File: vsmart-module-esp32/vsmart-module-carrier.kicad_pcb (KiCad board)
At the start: 2 copper layers, 105 x 82 mm, 12 parts, among them J1 EXTERNAL 5V INPUT, J2 EXTERNAL 5V 2A SIM INPUT, U1 ESP32-DevKitC 38-pin, U2 MPU6050 GY-521 MODULE, U3 GPS NEO-7M GY-GPSU3, U4 A7680C TDM2309 4G

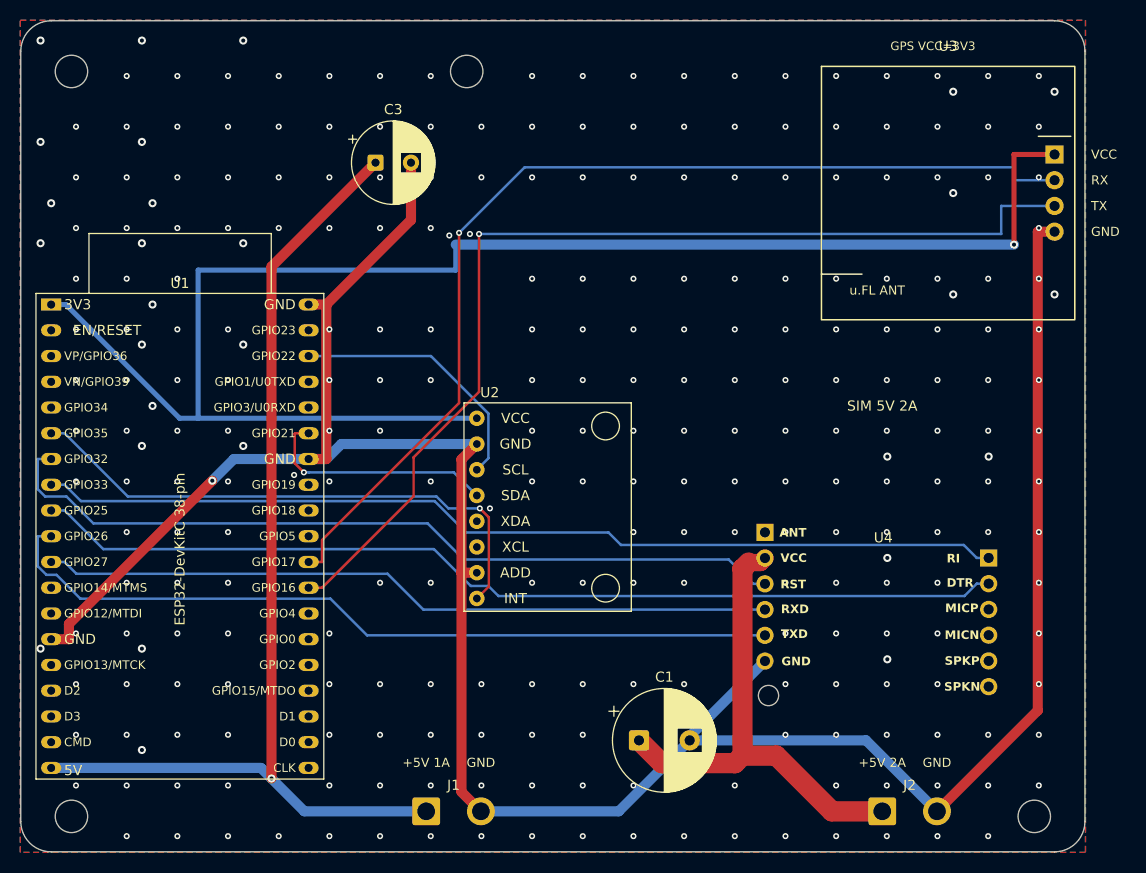
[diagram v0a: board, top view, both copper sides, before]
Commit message: chore: sync full workspace source into monorepo
Push current state of all first-party Vsmart components (backend, web,
web mobile, infrastructure, firmware, hardware, osrm, module variants)
directly from the DATN working tree, which is now the root of this repo.

Excluded: DRC/audit/build reports, auto-generated PCB snapshots, OSRM map
data, dependencies (node_modules/.venv/Pods/.pio), device secrets/certs,
.env files, local agent tooling, and vendored third-party reference repos
(ESP32_OSM_NAV, AWS guidance sample) per CLAUDE.md.

Co-Authored-By: Claude Sonnet 5 <noreply@anthropic.com>
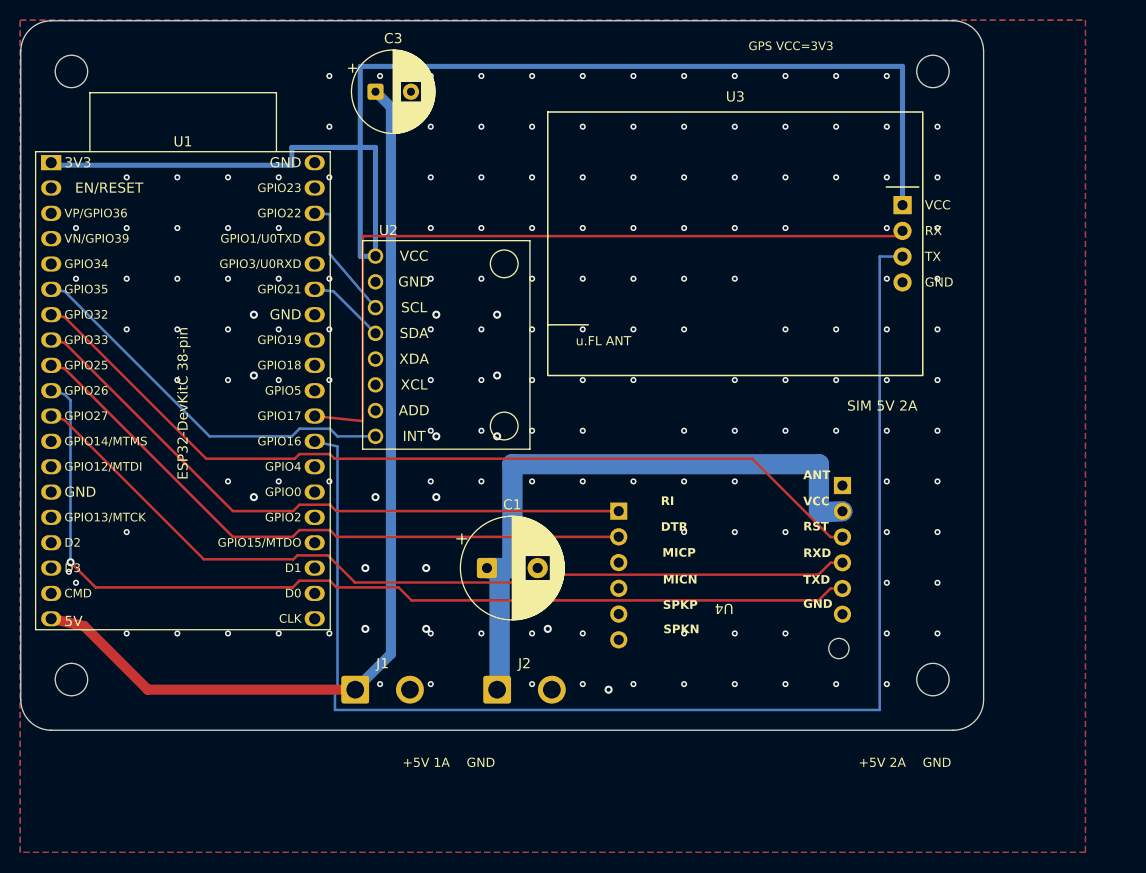
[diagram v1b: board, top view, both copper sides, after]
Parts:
- moved MH2 46.0 mm to (110.0, 25.0)
- moved J2 39.8 mm to (67.0, 86.0)
- moved U4 36.6 mm to (79.0, 76.0), turned to 180 degrees
- moved C1 22.7 mm to (66.0, 74.0)
- moved U2 18.9 mm to (55.0, 61.0)
- moved MH4 16.8 mm to (110.0, 85.0)
- moved U3 15.8 mm to (107.0, 42.0)
- moved U1 14.0 mm to (23.0, 34.0)
- moved J1 13.9 mm to (53.0, 86.0)
- moved MH3 13.5 mm to (25.0, 85.0)
- moved C3 7.00 mm to (55.0, 27.0)
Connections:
- U1 pad 5: GPS_PPS -> (no net)
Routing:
- net GND: track 250.9 -> 0.00 mm, vias 289 -> 171
- net SIM_DTR: track 96.5 -> 63.5 mm
- net SIM_RI: track 95.5 -> 63.4 mm
- net GPS_RX: track 102.2 -> 129.3 mm, vias 1 -> 0
- net GPS_TX: track 102.1 -> 76.8 mm, vias 1 -> 0
- net +3V3: track 157.2 -> 132.2 mm, vias 1 -> 0
- net SIM_RX: track 78.9 -> 96.9 mm, vias 0 -> 1
- net MPU_INT: track 55.3 -> 38.6 mm, vias 1 -> 0
- net I2C_SDA: track 23.6 -> 7.73 mm, vias 1 -> 0
- net +5V_SIM: track 48.6 -> 63.6 mm
- net I2C_SCL: track 26.1 -> 12.4 mm
- net SIM_TX: track 72.4 -> 85.9 mm
- net +5V: track 103.8 -> 93.8 mm, vias 1 -> 0
- net SIM_RST: track 79.9 -> 87.5 mm
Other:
- board size 105 x 82 mm -> 95 x 70 mm
